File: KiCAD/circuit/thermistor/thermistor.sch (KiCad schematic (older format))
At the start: 4 parts, among them J1 Conn_01x04_Male, J2 Conn_01x04_Male

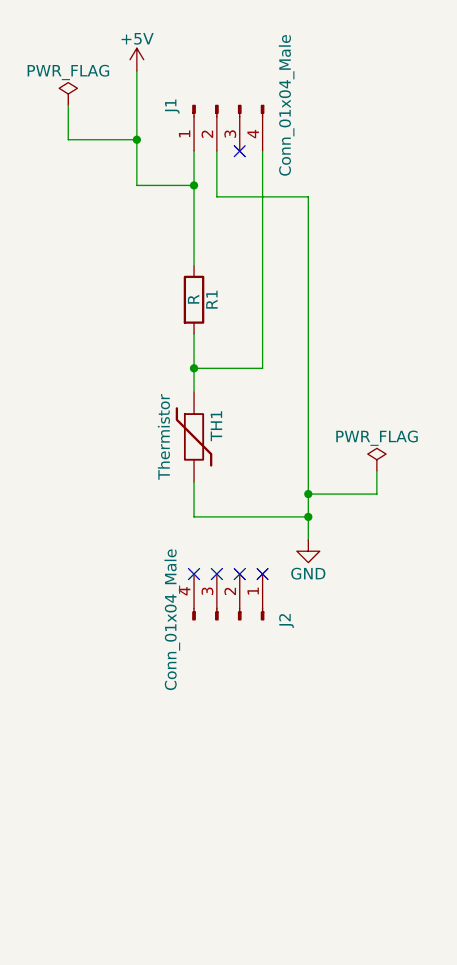
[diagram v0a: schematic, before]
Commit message: update
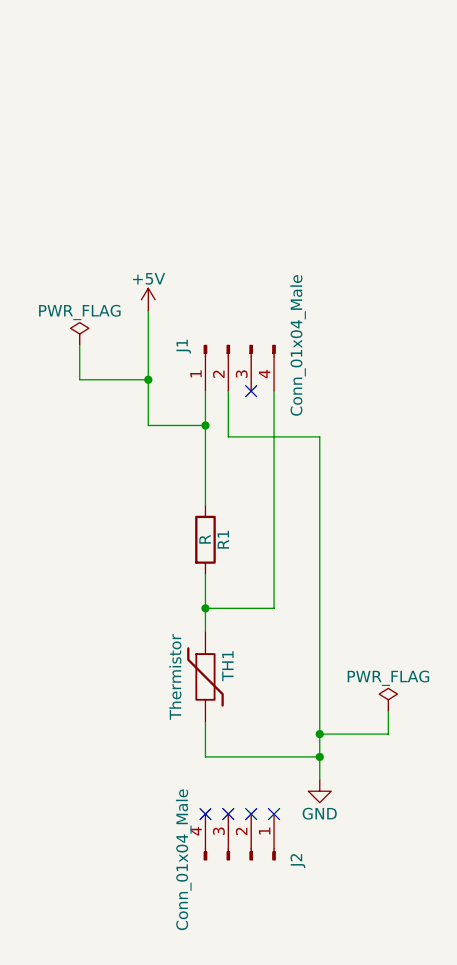
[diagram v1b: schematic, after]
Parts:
- J1, J2: footprint (none) -> can-bus:PinHeader_1x4
- R1: footprint (none) -> can-bus:Resistor_FaithfulLink_CF25
- TH1: footprint (none) -> can-bus:Thermistor
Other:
- moved on the sheet: J1, J2, R1, TH1
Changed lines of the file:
@@
 $EndDescr
 $Comp
-L +5V #PWR1
+L +5V #PWR01
 U 1 1 5AD6958B
-P 5150 1500
-F 0 "#PWR1" H 5150 1350 50  0001 C CNN
-F 1 "+5V" H 5150 1640 50  0000 C CNN
-F 2 "" H 5150 1500 50  0001 C CNN
-F 3 "" H 5150 1500 50  0001 C CNN
-	1    5150 1500
+P 5200 2550
+F 0 "#PWR01" H 5200 2400 50  0001 C CNN
+F 1 "+5V" H 5200 2690 50  0000 C CNN
+F 2 "" H 5200 2550 50  0001 C CNN
+F 3 "" H 5200 2550 50  0001 C CNN
+	1    5200 2550
 	1    0    0    -1
 $EndComp
@@
 L R R1
 U 1 1 5AD695C2
-P 5400 2500
-F 0 "R1" V 5480 2500 50  0000 C CNN
-F 1 "R" V 5400 2500 50  0000 C CNN
-F 2 "" V 5330 2500 50  0001 C CNN
-F 3 "" H 5400 2500 50  0001 C CNN
-	1    5400 2500
+P 5450 3550
+F 0 "R1" V 5530 3550 50  0000 C CNN
+F 1 "R" V 5450 3550 50  0000 C CNN
+F 2 "can-bus:Resistor_FaithfulLink_CF25" V 5380 3550 50  0001 C CNN
+F 3 "" H 5450 3550 50  0001 C CNN
+	1    5450 3550
 	1    0    0    -1
 $EndComp
@@
 L Thermistor TH1
 U 1 1 5AD695FB
-P 5400 3100
-F 0 "TH1" V 5500 3150 50  0000 C CNN
-F 1 "Thermistor" V 5300 3100 50  0000 C BNN
-F 2 "" H 5400 3100 50  0001 C CNN
-F 3 "" H 5400 3100 50  0001 C CNN
-	1    5400 3100
+P 5450 4150
+F 0 "TH1" V 5550 4200 50  0000 C CNN
+F 1 "Thermistor" V 5350 4150 50  0000 C BNN
+F 2 "can-bus:Thermistor" H 5450 4150 50  0001 C CNN
+F 3 "" H 5450 4150 50  0001 C CNN
+	1    5450 4150
 	1    0    0    -1
 $EndComp
@@
 L Conn_01x04_Male J1
 U 1 1 5AD696BC
-P 5500 1650
-F 0 "J1" H 5500 1850 50  0000 C CNN
-F 1 "Conn_01x04_Male" H 5500 1350 50  0000 C CNN
-F 2 "" H 5500 1650 50  0001 C CNN
-F 3 "" H 5500 1650 50  0001 C CNN
-	1    5500 1650
+P 5550 2700
+F 0 "J1" H 5550 2900 50  0000 C CNN
+F 1 "Conn_01x04_Male" H 5550 2400 50  0000 C CNN
+F 2 "can-bus:PinHeader_1x4" H 5550 2700 50  0001 C CNN
+F 3 "" H 5550 2700 50  0001 C CNN
+	1    5550 2700
 	0    -1   1    0
 $EndComp
@@
 L Conn_01x04_Male J2
 U 1 1 5AD696F6
-P 5600 3900
-F 0 "J2" H 5600 4100 50  0000 C CNN
-F 1 "Conn_01x04_Male" H 5600 3600 50  0000 C CNN
-F 2 "" H 5600 3900 50  0001 C CNN
-F 3 "" H 5600 3900 50  0001 C CNN
-	1    5600 3900
+P 5650 4950
+F 0 "J2" H 5650 5150 50  0000 C CNN
+F 1 "Conn_01x04_Male" H 5650 4650 50  0000 C CNN
+F 2 "can-bus:PinHeader_1x4" H 5650 4950 50  0001 C CNN
+F 3 "" H 5650 4950 50  0001 C CNN
+	1    5650 4950
 	0    1    -1   0
 $EndComp
 $Comp
-L GND #PWR2
+L GND #PWR02
 U 1 1 5AD6B029
-P 5900 3550
-F 0 "#PWR2" H 5900 3300 50  0001 C CNN
-F 1 "GND" H 5900 3400 50  0000 C CNN
-F 2 "" H 5900 3550 50  0001 C CNN
-F 3 "" H 5900 3550 50  0001 C CNN
-	1    5900 3550
+P 5950 4600
+F 0 "#PWR02" H 5950 4350 50  0001 C CNN
+F 1 "GND" H 5950 4450 50  0000 C CNN
+F 2 "" H 5950 4600 50  0001 C CNN
+F 3 "" H 5950 4600 50  0001 C CNN
+	1    5950 4600
 	1    0    0    -1
 $EndComp
 Wire Wire Line
-	5500 1850 5500 2050
+	5550 2900 5550 3100
 Wire Wire Line
-	5500 2050 5900 2050
+	5550 3100 5950 3100
 Wire Wire Line
-	5900 2050 5900 3550
+	5950 3100 5950 4600
 Wire Wire Line
-	5150 1500 5150 2000
+	5200 2550 5200 3050
 Wire Wire Line
-	5150 2000 5400 2000
+	5200 3050 5450 3050
 Wire Wire Line
-	5400 1850 5400 2350
+	5450 2900 5450 3400
 $Comp
-L PWR_FLAG #FLG1
+L PWR_FLAG #FLG03
 U 1 1 5AD6B0C5
-P 4850 1650
-F 0 "#FLG1" H 4850 1725 50  0001 C CNN
-F 1 "PWR_FLAG" H 4850 1800 50  0000 C CNN
-F 2 "" H 4850 1650 50  0001 C CNN
-F 3 "" H 4850 1650 50  0001 C CNN
-	1    4850 1650
+P 4900 2700
+F 0 "#FLG03" H 4900 2775 50  0001 C CNN
+F 1 "PWR_FLAG" H 4900 2850 50  0000 C CNN
+F 2 "" H 4900 2700 50  0001 C CNN
+F 3 "" H 4900 2700 50  0001 C CNN
+	1    4900 2700
 	1    0    0    -1
 $EndComp
 $Comp
-L PWR_FLAG #FLG2
+L PWR_FLAG #FLG04
 U 1 1 5AD6B0E1
-P 6200 3250
-F 0 "#FLG2" H 6200 3325 50  0001 C CNN
-F 1 "PWR_FLAG" H 6200 3400 50  0000 C CNN
-F 2 "" H 6200 3250 50  0001 C CNN
-F 3 "" H 6200 3250 50  0001 C CNN
-	1    6200 3250
+P 6250 4300
+F 0 "#FLG04" H 6250 4375 50  0001 C CNN
+F 1 "PWR_FLAG" H 6250 4450 50  0000 C CNN
+F 2 "" H 6250 4300 50  0001 C CNN
+F 3 "" H 6250 4300 50  0001 C CNN
+	1    6250 4300
 	1    0    0    -1
 $EndComp
 Wire Wire Line
-	4850 1650 4850 1800
+	4900 2700 4900 2850
 Wire Wire Line
-	4850 1800 5150 1800
-Connection ~ 5150 1800
+	4900 2850 5200 2850
+Connection ~ 5200 2850
 Wire Wire Line
-	5900 3350 6200 3350
+	5950 4400 6250 4400
 Wire Wire Line
-	6200 3350 6200 3250
-Connection ~ 5900 3350
-Connection ~ 5400 2000
+	6250 4400 6250 4300
+Connection ~ 5950 4400
+Connection ~ 5450 3050
 Wire Wire Line
-	5400 2650 5400 2900
+	5450 3700 5450 3950
 Wire Wire Line
-	5700 1850 5700 2800
+	5750 2900 5750 3850
 Wire Wire Line
-	5700 2800 5400 2800
-Connection ~ 5400 2800
+	5750 3850 5450 3850
+Connection ~ 5450 3850
 Wire Wire Line
-	5400 3300 5400 3450
+	5450 4350 5450 4500
 Wire Wire Line
-	5400 3450 5900 3450
-Connection ~ 5900 3450
-NoConn ~ 5600 1850
-NoConn ~ 5400 3700
-NoConn ~ 5500 3700
-NoConn ~ 5600 3700
-NoConn ~ 5700 3700
+	5450 4500 5950 4500
+Connection ~ 5950 4500
+NoConn ~ 5650 2900
+NoConn ~ 5450 4750
+NoConn ~ 5550 4750
+NoConn ~ 5650 4750
+NoConn ~ 5750 4750
 $EndSCHEMATC
